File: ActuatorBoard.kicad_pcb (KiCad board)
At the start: 2 copper layers, 75 x 89.5 mm, 84 parts, among them J1 Screw_Terminal_01x02, J11 Screw_Terminal_01x02, J12 Screw_Terminal_01x02, J13 Screw_Terminal_01x04, J2 Screw_Terminal_01x02, J3 Screw_Terminal_01x02, J4 Screw_Terminal_01x02, J5 Screw_Terminal_01x02, J7 Screw_Terminal_01x02, J8 Screw_Terminal_01x02, J9 Screw_Terminal_01x02, K1 SANYOU_SRD_Form_B, K2 SANYOU_SRD_Form_B, K3 SANYOU_SRD_Form_B, P1 CONN_01X03, P10 CONN_01X03, P11 CONN_01X03, P12 CONN_01X03, P13 CONN_01X02, P14 SERVO_+, P15 SERVO_-, P16 CONN_01X03, P17 CONN_01X05, P18 CONN_01X08, P19 CONN_01X05, P2 CAN_Conn, P20 CONN_01X08, P21 STEPPER_VCC, P22 CONN_01X05, P23 CONN_01X04, P3 CONN_01X03, P4 CONN_01X03, P5 CONN_01X03, P6 CONN_01X06, P7 CONN_01X03, P8 CONN_01X03, P9 CONN_01X03, Q1 BS170, Q2 BS170, Q3 BS170, Q5 IRLR024, U1 MCP2551-I-SN, U2 AT90CAN128-16AU, U3 ULN2003, U4 L7805, Y1 Crystal, Y2 Crystal

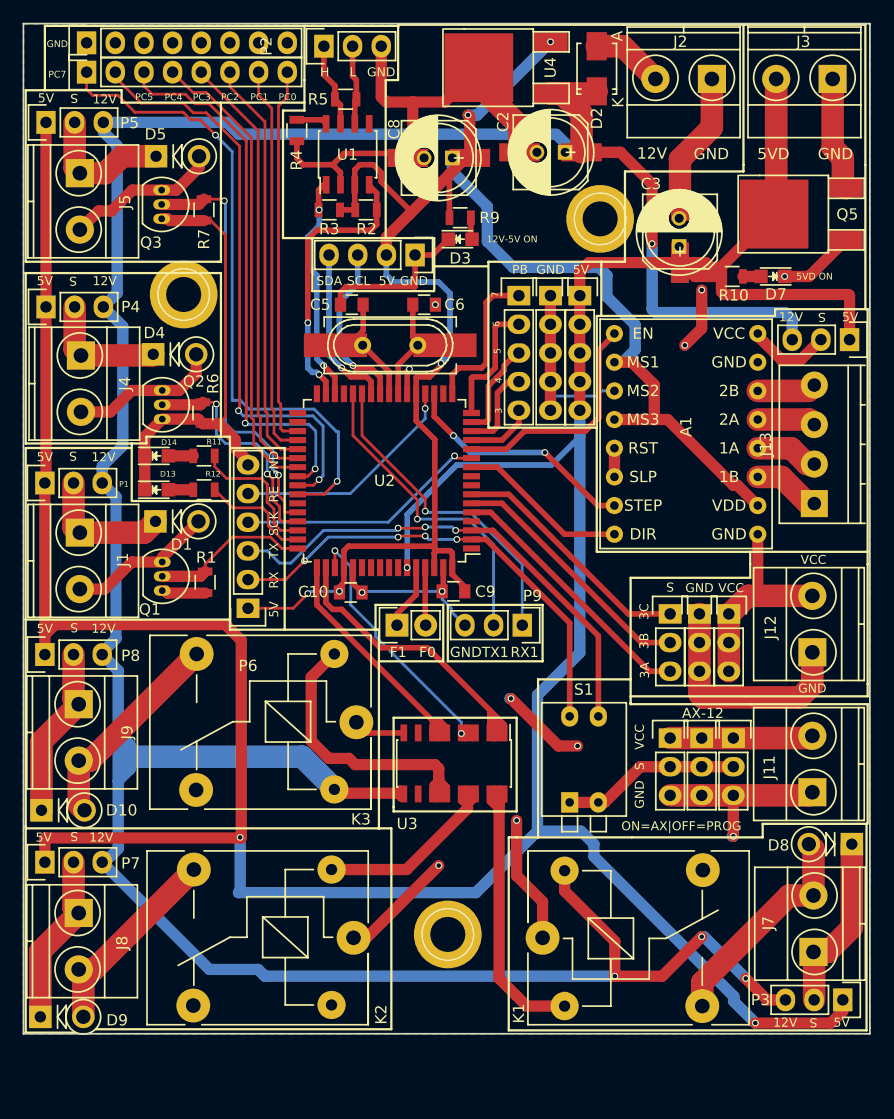
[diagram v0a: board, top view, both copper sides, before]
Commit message: Actuator board with modules
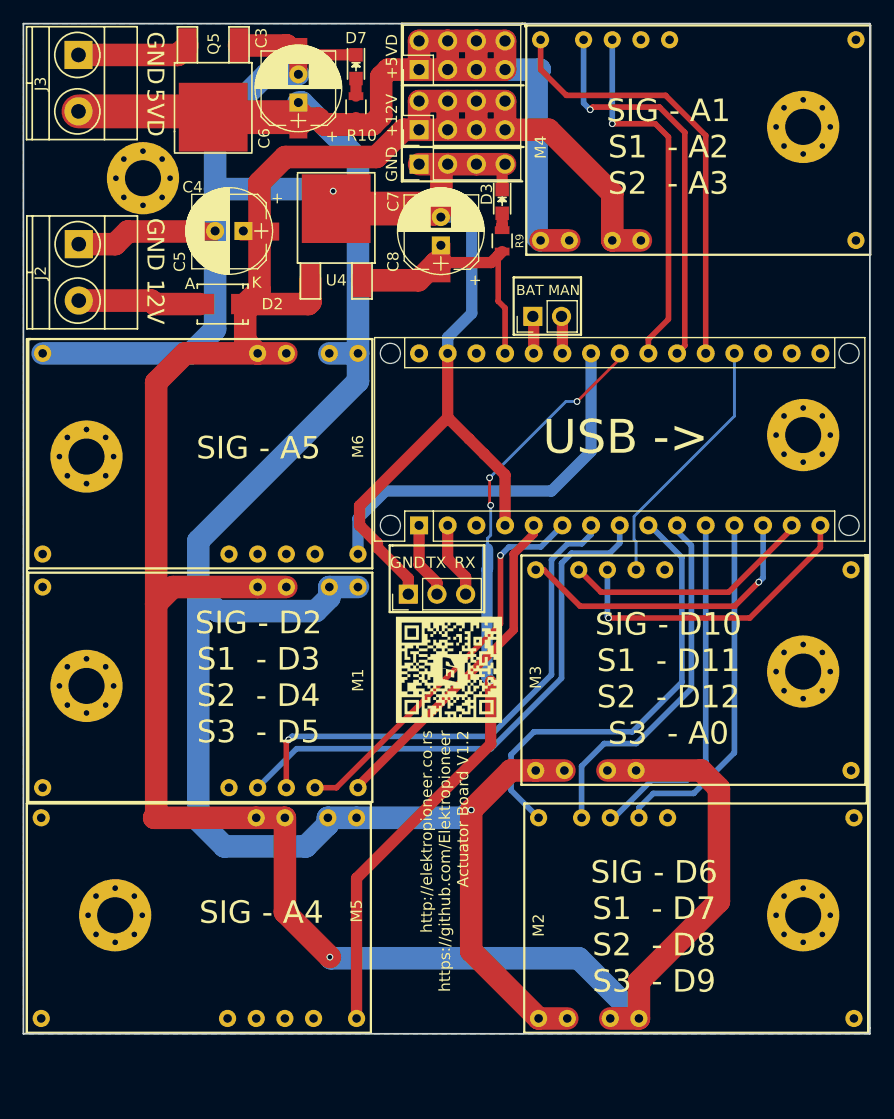
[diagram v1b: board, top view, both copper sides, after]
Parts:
- removed A1: Pololu_Breakout_A4988, A4988:A4988
- removed C1, C2: 100u, Capacitors_ThroughHole:C_Radial_D7.5_L11.2_P2.5
- removed C10, C9: 100n, Capacitors_SMD:C_0805
- removed D1, D10, D4, D5, D8, D9: D, Diodes_ThroughHole:Diode_DO-41_SOD81_Vertical_KathodeUp
- removed D13, D14: LED, LEDs:LED_0805
- removed J11, J12, J7, J8, J9: Screw_Terminal_01x02, Terminal_Blocks:TerminalBlock_Pheonix_MKDS1.5-2pol
- removed J13: Screw_Terminal_01x04, Terminal_Blocks:TerminalBlock_Pheonix_PT-3.5mm_4pol
- removed K1, K2, K3: SANYOU_SRD_Form_B, Relays_ThroughHole:Relay_SANYOU_SRD_Series_Form_C
- removed P10, P11, P12, P16, P3, P4, P5, P7, P8, P9: CONN_01X03, Pin_Headers:Pin_Header_Straight_1x03
- removed P14: SERVO_+, Pin_Headers:Pin_Header_Straight_1x03
- removed P15: SERVO_-, Pin_Headers:Pin_Header_Straight_1x03
- removed P17, P19, P22: CONN_01X05, Pin_Headers:Pin_Header_Straight_1x05
- removed P18, P20: CONN_01X08, Pin_Headers:Pin_Header_Straight_1x08
- removed P2: CAN_Conn, Pin_Headers:Pin_Header_Straight_1x03
- removed P21: STEPPER_VCC, Pin_Headers:Pin_Header_Straight_1x03
- removed P23: CONN_01X04, Pin_Headers:Pin_Header_Straight_1x04
- removed P6: CONN_01X06, Pin_Headers:Pin_Header_Straight_1x06
- removed Q1, Q2, Q3: BS170, TO_SOT_Packages_THT:TO-92_Inline_Narrow_Oval
- removed R1, R6, R7: R, Resistors_SMD:R_0805
- removed R11, R12: 330, Resistors_SMD:R_0805
- removed R2, R3: 1K, Resistors_SMD:R_0805
- removed R4: 10K, Resistors_SMD:R_0805
- removed R5: 120, Resistors_SMD:R_0805
- removed REF** (x3): 1pin, Connect:1pin
- removed S1: SW_DIP_x2, Buttons_Switches_ThroughHole:SW_DIP_x2_Piano
- removed U1: MCP2551-I-SN, Housings_SOIC:SOIC-8_3.9x4.9mm_Pitch1.27mm
- removed U2: AT90CAN128-16AU, Housings_QFP:TQFP-64_14x14mm_Pitch0.8mm
- removed U3: ULN2003, Housings_SOIC:SOIC-16_3.9x9.9mm_Pitch1.27mm
- removed Y1: Crystal, Crystals:Crystal_HC49-SD_SMD
- removed Y2: Crystal, Crystals:Crystal_HC49-U_Vertical
- added A2: Arduino_Nano_v3.x, Modules:Arduino_Nano_WithMountingHoles, F.Cu at (196.6, 69.0)
- added G***: LOGO, Hardware:EP_Logo, F.Cu at (199.2, 81.8)
- added G***: LOGO, Hardware:EP_Logo_2, B.Cu at (225.9, 43.8)
- added G***: LOGO, Hardware:github_logo, B.Cu at (189.2, 43.8)
- added M1: Aktuator_Module, Aktuator_Module:Aktuator_Module, F.Cu at (192.4, 93.5)
- added M2: Aktuator_Module, Aktuator_Module:Aktuator_Module, F.Cu at (205.9, 93.6)
- added M3: Aktuator_Module, Aktuator_Module:Aktuator_Module, F.Cu at (205.6, 71.6)
- added M4: Aktuator_Module, Aktuator_Module:Aktuator_Module, F.Cu at (206.1, 24.7)
- added M5: Aktuator_Module, Aktuator_Module:Aktuator_Module, F.Cu at (192.3, 113.9)
- added M6: Aktuator_Module, Aktuator_Module:Aktuator_Module, F.Cu at (192.4, 72.8)
- added MK1: Mounting_Hole, Mounting_Holes:MountingHole_3.2mm_M3_Pad_Via, F.Cu at (172.1, 38.2)
- added MK2: Mounting_Hole, Mounting_Holes:MountingHole_3.2mm_M3_Pad_Via, F.Cu at (230.6, 103.5)
- added MK3: Mounting_Hole, Mounting_Holes:MountingHole_3.2mm_M3_Pad_Via, F.Cu at (230.6, 81.9)
- added MK4: Mounting_Hole, Mounting_Holes:MountingHole_3.2mm_M3_Pad_Via, F.Cu at (169.6, 103.5)
- added MK5: Mounting_Hole, Mounting_Holes:MountingHole_3.2mm_M3_Pad_Via, F.Cu at (167.1, 83.2)
- added MK6: Mounting_Hole, Mounting_Holes:MountingHole_3.2mm_M3_Pad_Via, F.Cu at (167.1, 62.9)
- added MK7: Mounting_Hole, Mounting_Holes:MountingHole_3.2mm_M3_Pad_Via, F.Cu at (230.6, 33.6)
- added MK8: Mounting_Hole, Mounting_Holes:MountingHole_3.2mm_M3_Pad_Via, F.Cu at (230.6, 61.0)
- added REF***: KiCad-Logo2_12mm_SilkScreen, Symbols:KiCad-Logo2_12mm_SilkScreen, B.Cu at (213.9, 60.8)
- C3, C4, C8: footprint Capacitors_SMD:c_elec_6.3x4.5 -> Capacitors_SMD:CP_Elec_6.3x4.5
- C5, C6: value C -> 100u; footprint Capacitors_SMD:C_0805 -> Capacitors_THT:CP_Radial_D7.5mm_P2.50mm
- C7: footprint Capacitors_ThroughHole:C_Radial_D7.5_L11.2_P2.5 -> Capacitors_THT:CP_Radial_D7.5mm_P2.50mm
- J1, J4: value Screw_Terminal_01x02 -> CONN_02X04; footprint Terminal_Blocks:TerminalBlock_Pheonix_MKDS1.5-2pol -> Pin_Headers:Pin_Header_Straight_2x04_Pitch2.54mm
- J2, J3: footprint Terminal_Blocks:TerminalBlock_Pheonix_MKDS1.5-2pol -> Connectors_Terminal_Blocks:TerminalBlock_Pheonix_MKDS1.5-2pol
- J5: value Screw_Terminal_01x02 -> CONN_01X03; footprint Terminal_Blocks:TerminalBlock_Pheonix_MKDS1.5-2pol -> Pin_Headers:Pin_Header_Straight_1x03_Pitch2.54mm
- P1: value CONN_01X03 -> CONN_01X04; footprint Pin_Headers:Pin_Header_Straight_1x03 -> Pin_Headers:Pin_Header_Straight_1x04_Pitch2.54mm
- P13: footprint Pin_Headers:Pin_Header_Straight_1x02 -> Pin_Headers:Pin_Header_Straight_1x02_Pitch2.54mm
- moved J3 66.9 mm to (166.4, 27.3), turned to 270 degrees
- moved Q5 58.0 mm to (178.3, 26.4), turned to 180 degrees
- moved J2 58.0 mm to (166.4, 44.0), turned to 270 degrees
- moved J5 47.3 mm to (195.6, 75.1), turned to 90 degrees
- moved J1 46.7 mm to (196.6, 33.9), turned to 90 degrees
- moved P1 43.6 mm to (196.6, 37.0)
- moved D7 41.3 mm to (191.0, 28.3), turned to 270 degrees
- moved J4 39.2 mm to (196.6, 28.6), turned to 90 degrees
- moved D2 39.2 mm to (179.2, 49.3), turned to 180 degrees
- moved R10 36.6 mm to (191.0, 31.9), turned to 90 degrees
- moved C3 36.1 mm to (185.9, 30.2), turned to 90 degrees
- moved P13 29.9 mm to (206.6, 50.4)
- moved C4 29.3 mm to (179.7, 42.9), turned to 180 degrees
- moved U4 26.7 mm to (189.2, 47.2), turned to 0 degrees
- moved C6 21.1 mm to (185.9, 31.5), turned to 90 degrees
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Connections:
- C3 pad 1: PF2 -> +5VD
- C5 pad 1: Net-(C5-Pad1) -> +12V
- C6 pad 1: Net-(C6-Pad1) -> +5VD
- J1 pad 1: Net-(D1-Pad1) -> +12V
- J1 pad 2: Net-(D1-Pad2) -> +12V
- J3 pad 2: PF2 -> +5VD
- J4 pad 1: Net-(D4-Pad1) -> +5VD
- J4 pad 2: Net-(D4-Pad2) -> +5VD
- J5 pad 1: Net-(D5-Pad1) -> GND
- J5 pad 2: Net-(D5-Pad2) -> TX
- P1 pad 1: PF2 -> GND
- P1 pad 2: Net-(D1-Pad1) -> GND
- P1 pad 3: +12V -> GND
- P13 pad 1: PF1 -> BAT_ODO_ADC
- P13 pad 2: PF0 -> BAT_MAIN_ADC
- Q5 pad 2: PF2 -> +5VD
- R10 pad 1: PF2 -> +5VD
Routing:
- net PF2: track 306.0 -> 0.00 mm, vias 3 -> 0
- net +5VD: track 0.00 -> 236.9 mm, vias 0 -> 1
- net +5V: track 158.3 -> 22.4 mm, vias 5 -> 0
- net GND: track 231.0 -> 157.5 mm, vias 12 -> 1
- net M_ADC_5: track 0.00 -> 69.5 mm, vias 0 -> 4
- net PC7: track 58.2 -> 0.00 mm, vias 2 -> 0
- net PC6: track 52.8 -> 0.00 mm, vias 2 -> 0
- net PC5: track 49.8 -> 0.00 mm, vias 2 -> 0
- net SIG4: track 0.00 -> 48.6 mm
- net SIG3: track 0.00 -> 45.4 mm, vias 0 -> 1
- net TX0: track 43.9 -> 0.00 mm, vias 3 -> 0
- net RX0: track 41.6 -> 0.00 mm, vias 4 -> 0
- net PC4: track 41.4 -> 0.00 mm
- net SIG5: track 0.00 -> 39.6 mm
- net M_ADC_2: track 0.00 -> 39.0 mm
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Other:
- board text added: "+12V"
- board text added: "+5VD"
- board text added: "BAT MAN"
- board text added: "SIG - A1 S1 - A2 S2 - A3"
- board text added: "SIG - A4"
- board text added: "SIG - A5"
- board text added: "SIG - D10 S1 - D11 S2 - D12 S3 - A0"
- board text added: "SIG - D2 S1 - D3 S2 - D4 S3 - D5"
- board text added: "SIG - D6 S1 - D7 S2 - D8 S3 - D9"
- board text added: "USB ->"
- board text added: "http://elektropioneer.co.rs https://github.com/Elektropioneer Actuator Board V1.2"
- board text removed: "12V-5V ON"
- board text removed: "3"
- board text removed: "3A"
- board text removed: "3B"
- board text removed: "3C"
- board text removed: "4"
- board text removed: "5"
- board text removed: "5V"
- board text removed: "5VD ON"
- board text removed: "6"
- board text removed: "7"
- board text removed: "AX-12"
- board text removed: "F0"
- board text removed: "F1"
- board text removed: "H"
- board text removed: "L"
- board text removed: "ON=AX|OFF=PROG"
- board text removed: "PB"
- board text removed: "PC0"
- board text removed: "PC1"
- board text removed: "PC2"
- board text removed: "PC3"
- board text removed: "PC4"
- board text removed: "PC5"
- board text removed: "PC7"
- board text removed: "RE"
- board text removed: "RX1"
- board text removed: "S"
- board text removed: "SCK"
- board text removed: "SCL"
- board text removed: "SDA"
- board text removed: "TX1"
- board text removed: "VCC"
- board text removed: "http://elektropioneer.co.rs/ https://github.com/Elektropioneer Actuator Board V1"

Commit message: Added outputs, pdf, screenshots
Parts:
- moved G*** 0.05 mm to (226.0, 43.8)
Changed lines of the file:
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@@
     (links 105)
     (no_connects 1)
-    (area 161.424999 24.424999 236.575001 114.075001)
+    (area 161.353799 21.146027 238.939001 114.364)
     (thickness 1.6)
     (drawings 49)
@@
   )
   (module Hardware:EP_Logo_2 (layer B.Cu)
-    (at 225.9164 43.7592 180)
+    (at 225.9672 43.7592 180)
     (fp_text reference G*** (at 0 0 180) (layer B.SilkS) hide
       (effects (font (thickness 0.3)) (justify mirror))
